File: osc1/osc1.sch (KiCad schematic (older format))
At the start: 48 parts

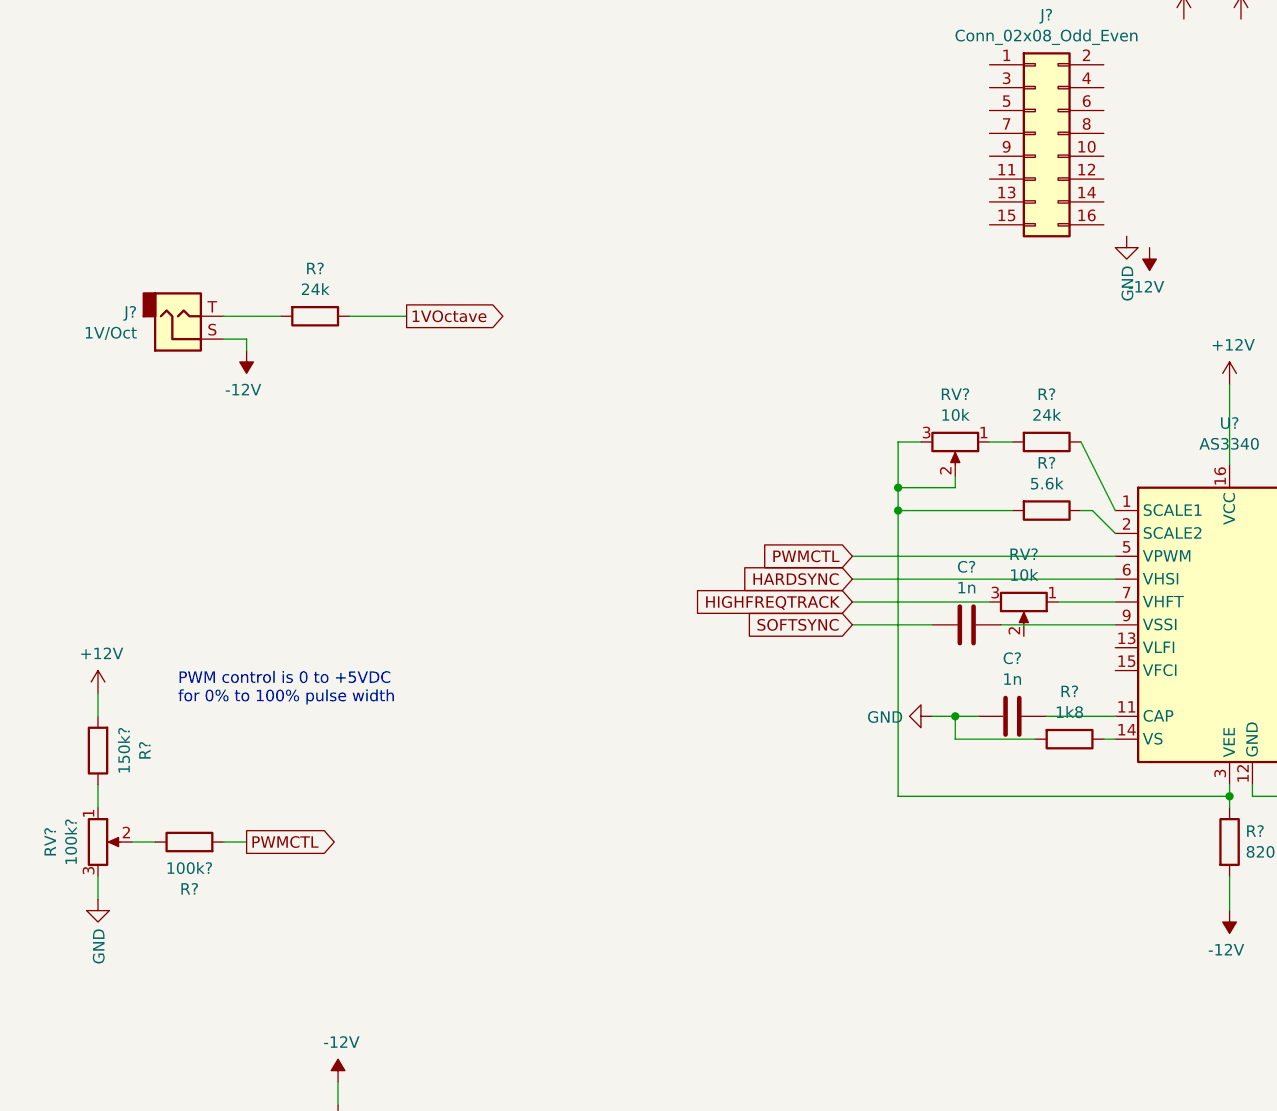
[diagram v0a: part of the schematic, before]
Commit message: Continued work on OSC1
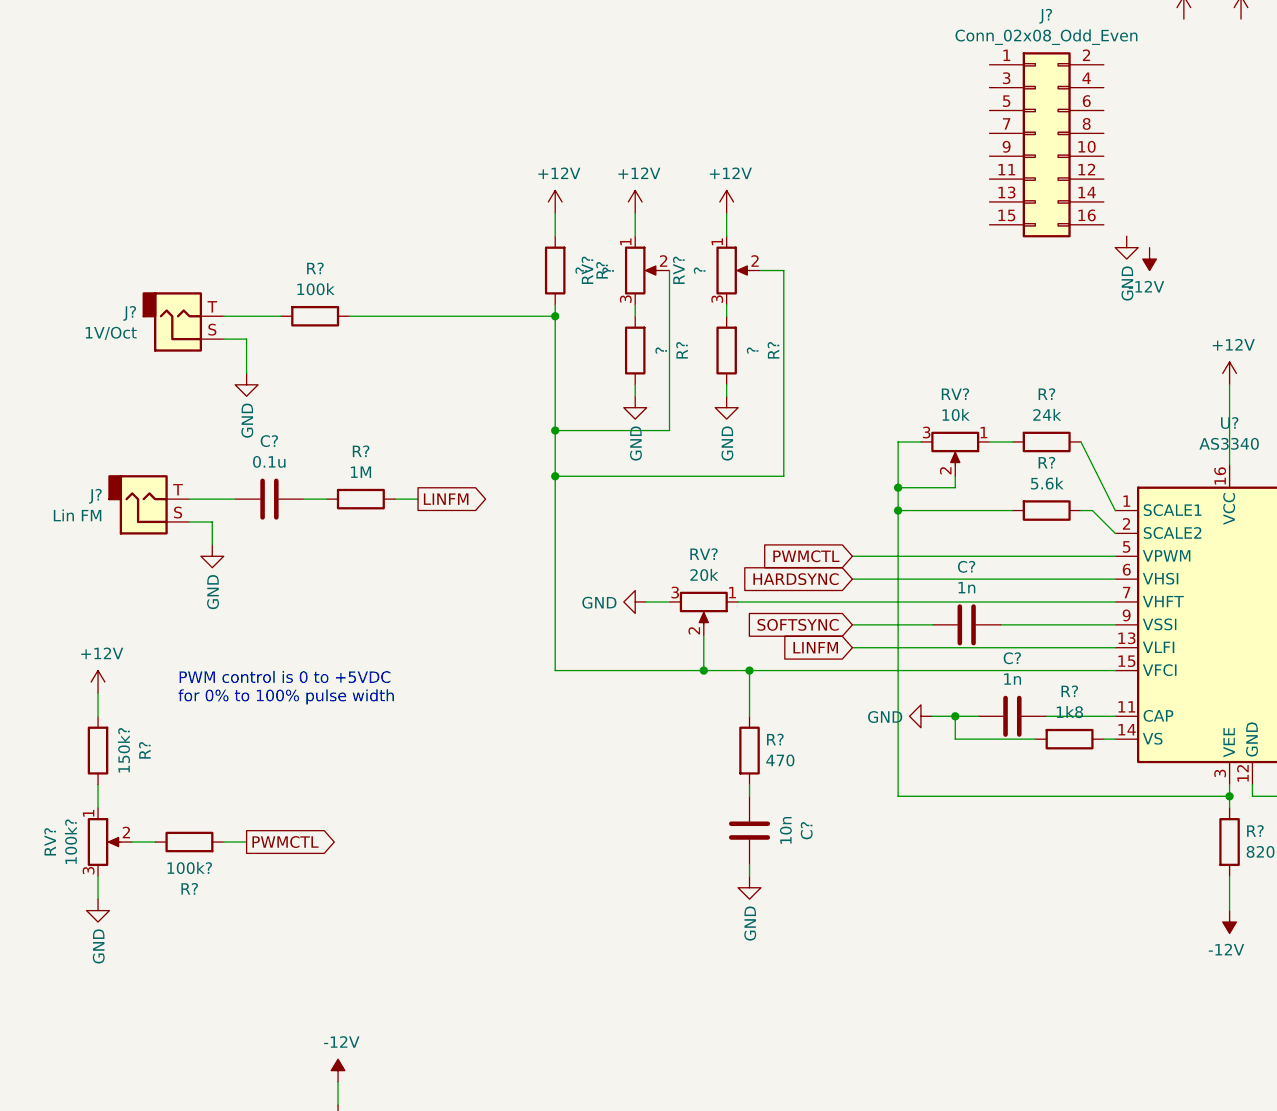
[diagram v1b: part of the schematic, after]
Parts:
- added C?: 0.1u, symbol Device:C
- added C?: 10n, symbol Device:C
- added J?: Lin FM, symbol Connector:AudioJack2
- added R?: 1M, symbol Device:R
- added R?: 470, symbol Device:R
- added R? (x3): ?, symbol Device:R
- added RV? (x2): ?, symbol Device:R_POT
- R?: value 24k -> 100k
- RV?: value 10k -> 20k
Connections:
- net 1VOctave is gone; now on an unnamed net: R?.1
- net HIGHFREQTRACK is gone; now on net GND: RV?.3
- net +12V: now also R?.2, RV?.1, RV?.1
- net -12V: no longer J?.S
- net GND: now also J?.S, C?.1, J?.S, R?.1, R?.1
- net LINFM: now reaches U?.13 (VLFI)
- net LINFM: now also R?.1
- net at U?.15 (VFCI): now also RV?.2, R?.1, R?.1, RV?.2, RV?.2
- new net: C?.2, J?.T
- new net: C?.1, R?.2
- new net: C?.2, R?.2
- new net: R?.2, RV?.3 (x2)
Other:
- moved on the sheet: RV?
